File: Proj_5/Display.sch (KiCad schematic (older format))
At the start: 10 parts, among them U15 74LVC1G11, U16 74LVC1G11, U26 74LVC1G11, U27 74LVC1G11, U28 74LVC1G11, U29 74LVC1G11, U30 74LVC1G11, U31 74LVC1G11, U32 PAL16L8

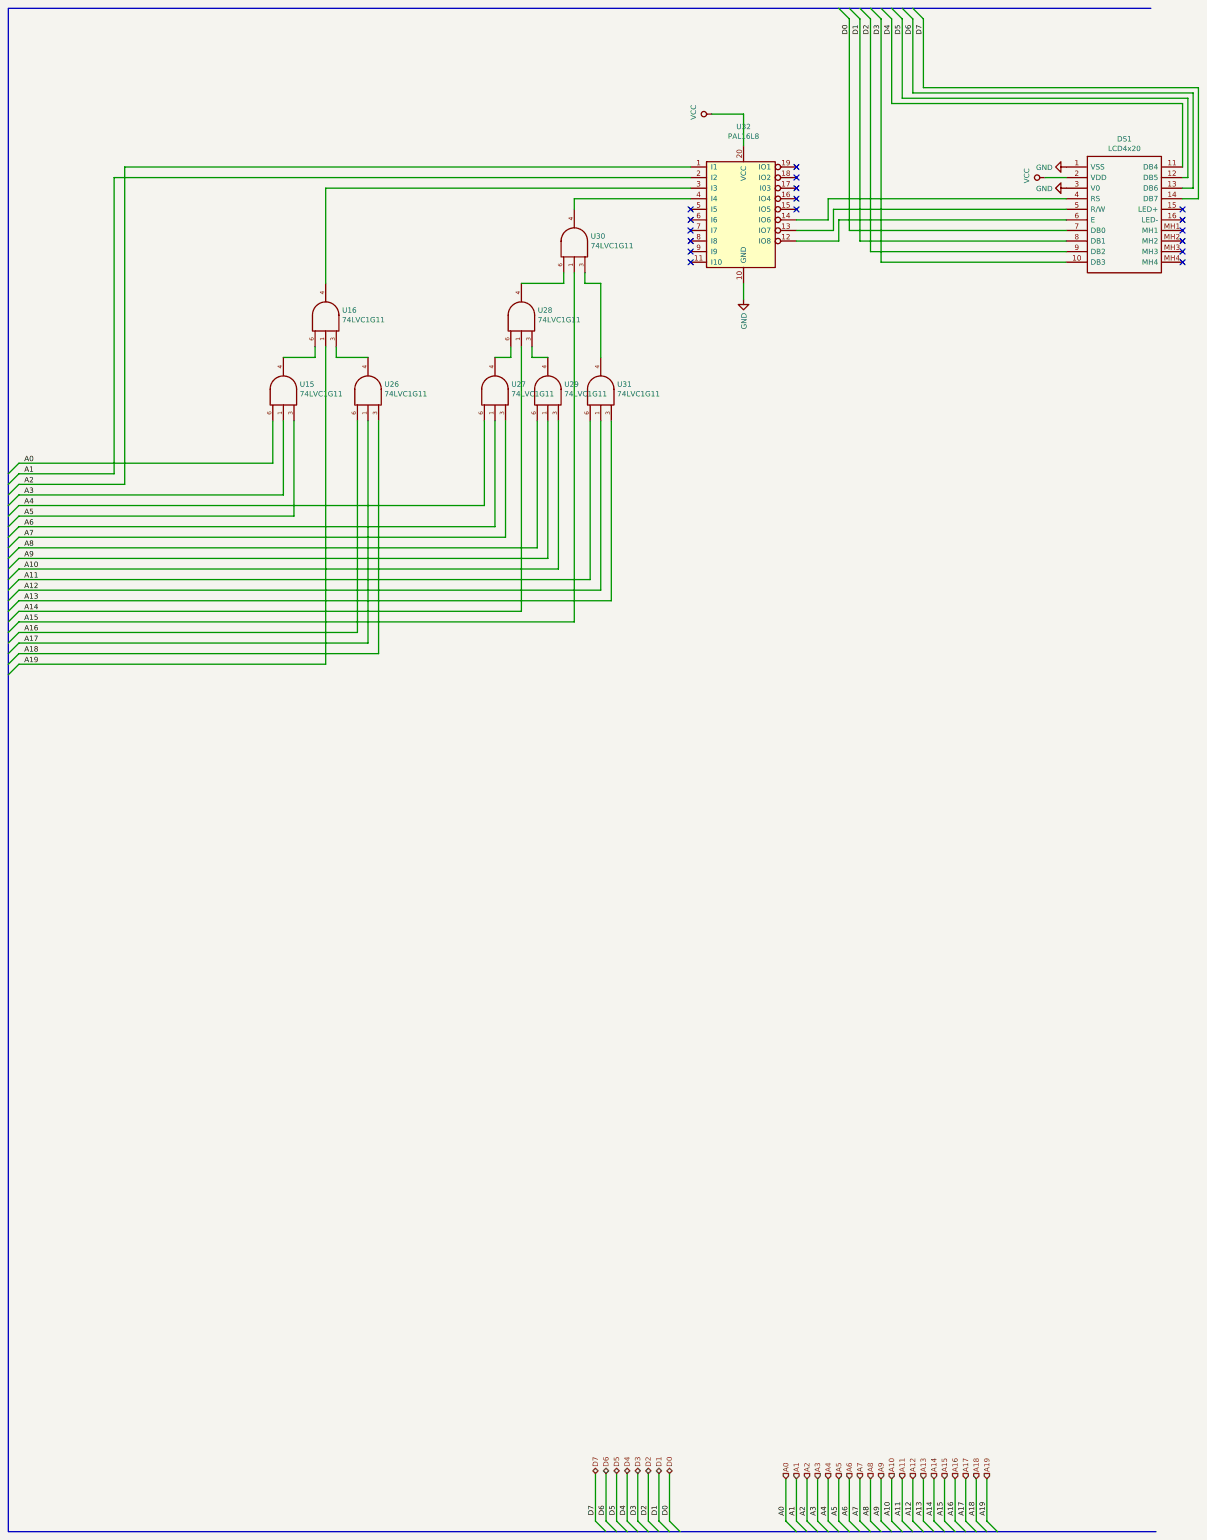
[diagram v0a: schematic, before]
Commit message: No more gates 2
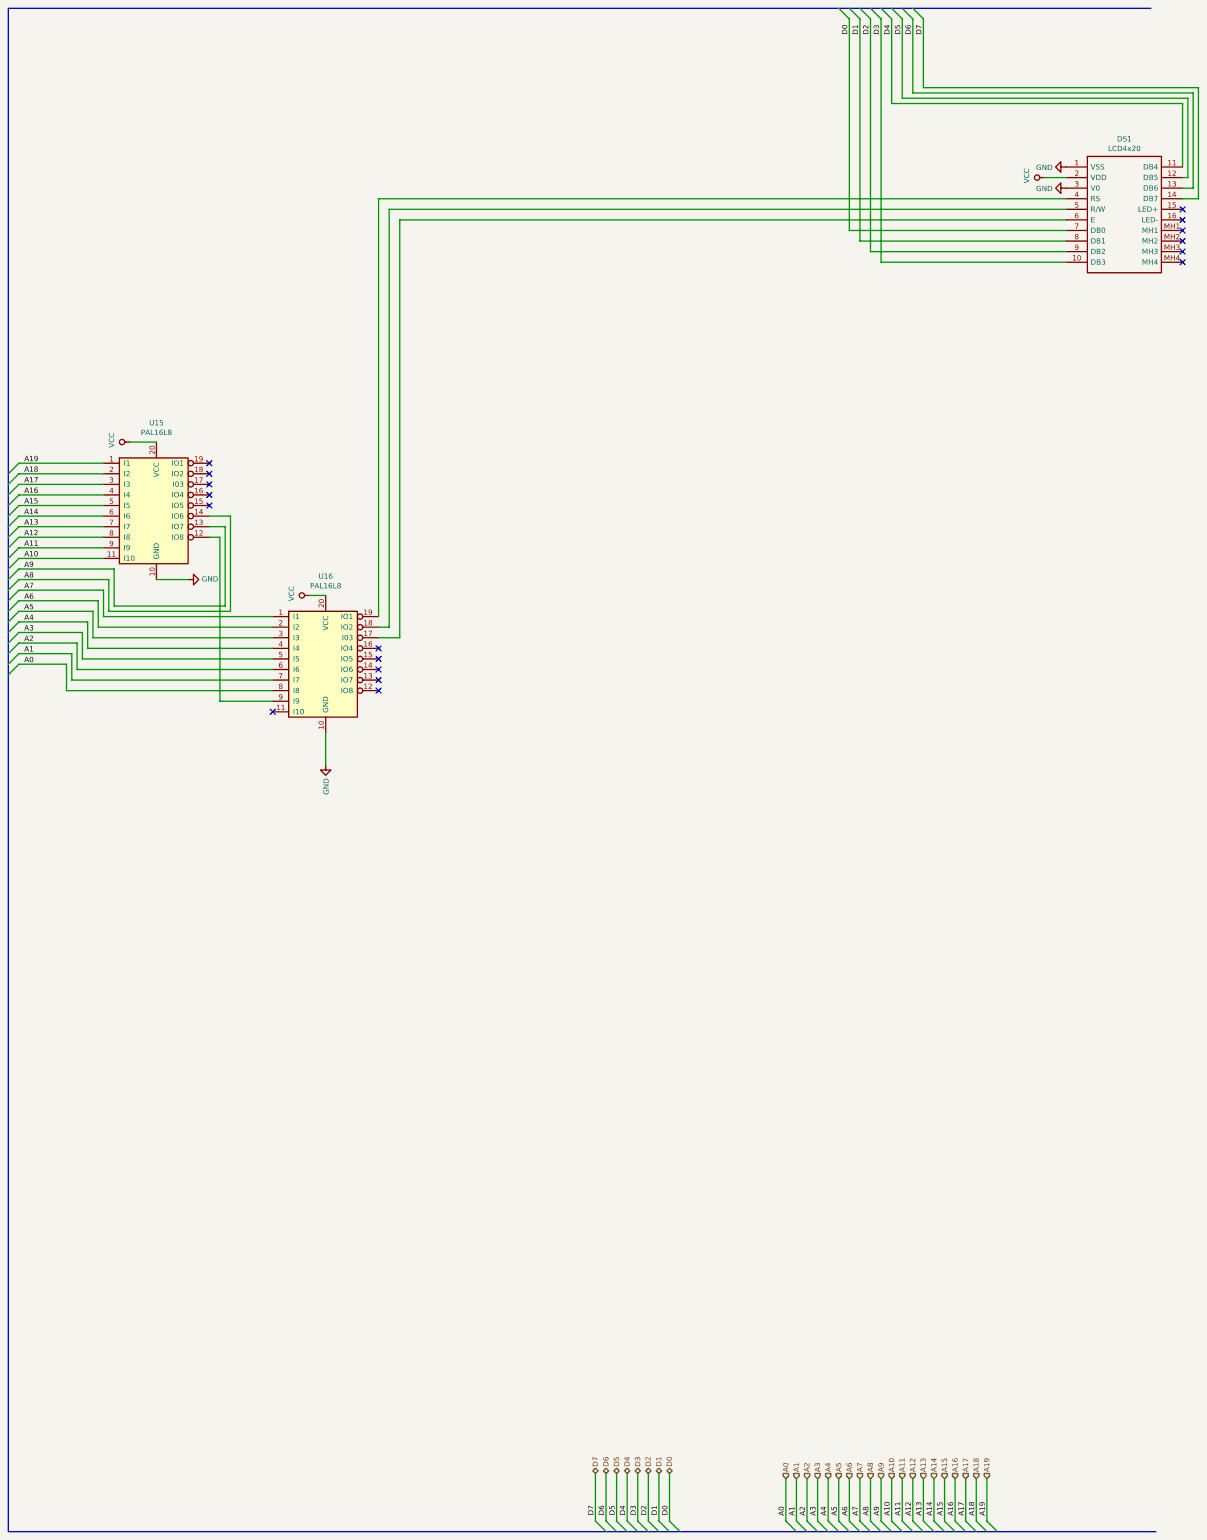
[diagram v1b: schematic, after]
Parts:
- removed U15, U16, U26, U27, U28, U29, U30, U31: 74LVC1G11, symbol 74xGxx:74LVC1G11
- removed U32: PAL16L8, Package_DIP:DIP-20_W7.62mm, symbol Logic_Programmable:PAL16L8
- added U15, U16: PAL16L8, Package_DIP:DIP-20_W7.62mm, symbol Logic_Programmable:PAL16L8
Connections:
- net A0: now also U16.8 (I8)
- net A1: now also U16.7 (I7)
- net A10: now also U15.11 (I10)
- net A11: now also U15.9 (I9)
- net A12: now also U15.8 (I8)
- net A13: now also U15.7 (I7)
- net A14: now also U15.6 (I6)
- net A15: now also U15.5 (I5)
- net A16: now also U15.4 (I4)
- net A17: now also U15.3 (I3)
- net A18: now also U15.2 (I2)
- net A19: now also U15.1 (I1)
- net A2: now also U16.6 (I6)
- net A3: now also U16.5 (I5)
- net A4: now also U16.4 (I4)
- net A5: now also U16.3 (I3)
- net A6: now also U16.2 (I2)
- net A7: now also U16.1 (I1)
- net A8: now also U15.14 (IO6)
- net A9: now also U15.13 (IO7)
- net GND: now also U15.10 (GND), U16.10 (GND)
- net VCC: now also U15.20 (VCC), U16.20 (VCC)
- net at DS1.6 (E): now also U16.17 (I03)
- net at DS1.5 (R/W): now also U16.18 (IO2)
- net at DS1.4 (RS): now also U16.19 (IO1)
- new net: U15.12 (IO8), U16.9 (I9)
